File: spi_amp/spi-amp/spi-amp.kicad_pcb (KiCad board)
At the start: 4 copper layers, 22.3 x 32.8 mm, 5 parts, among them J1 IN+, J2 IN-, J3 OUT+, J4 OUT-, U1 LMH6401

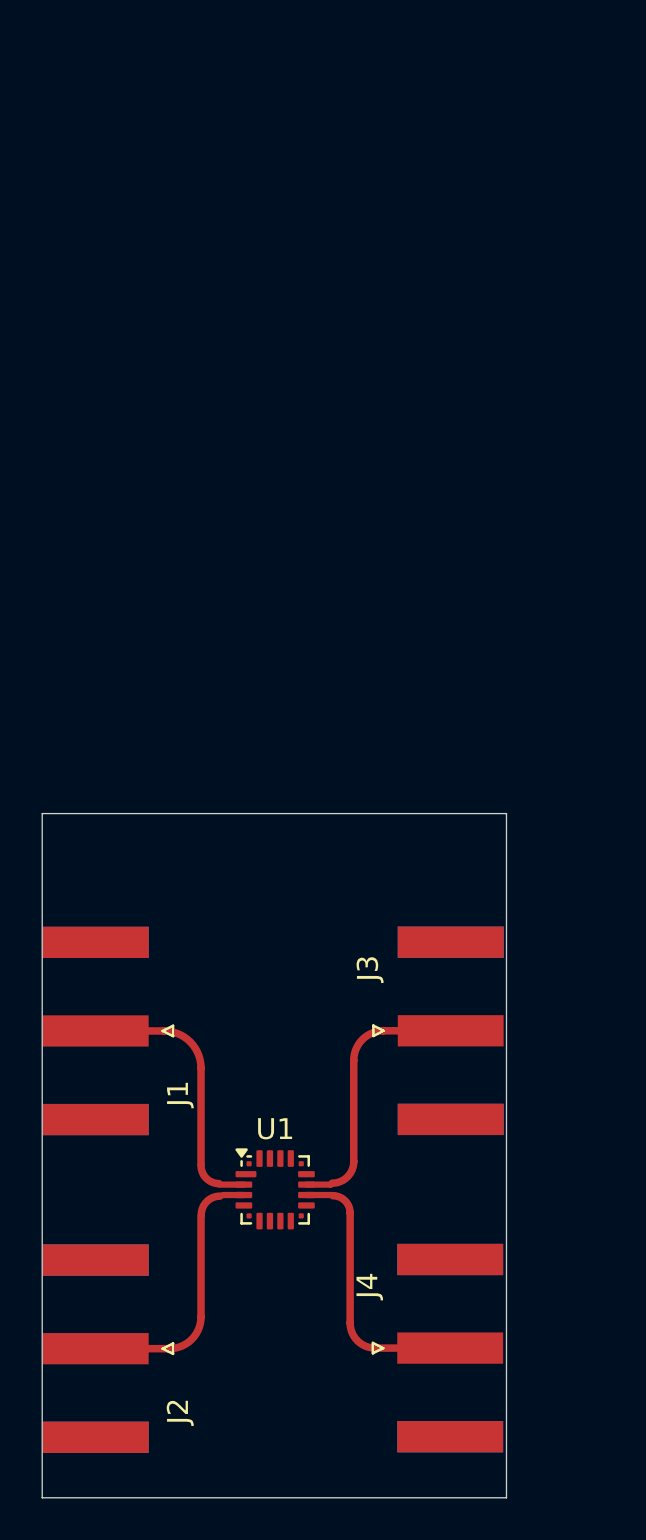
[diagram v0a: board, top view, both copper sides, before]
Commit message: Fixed layout for SPI RF PCB.
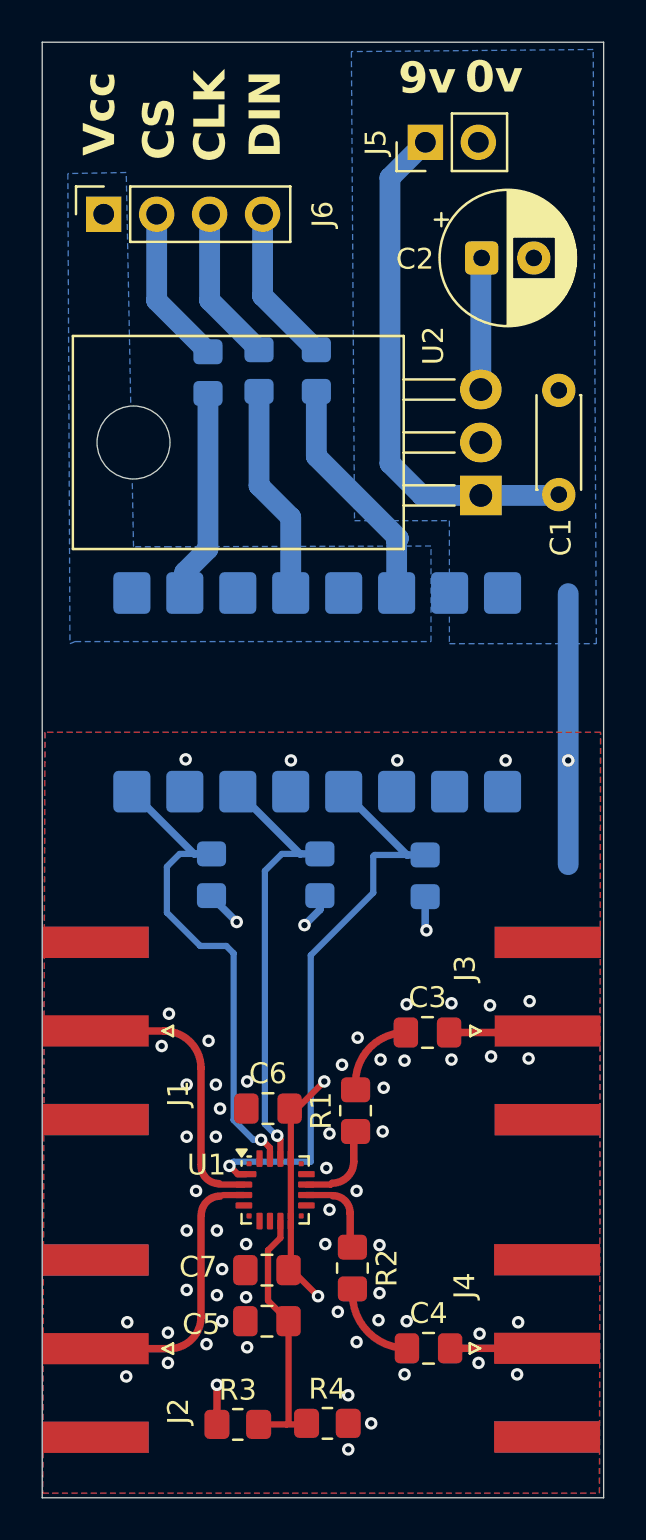
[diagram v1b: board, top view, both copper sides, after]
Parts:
- added C1: 47n, Capacitor_THT:C_Disc_D4.3mm_W1.9mm_P5.00mm, F.Cu at (130.7, 58.6)
- added C2: 22uF, Capacitor_THT:CP_Radial_D6.3mm_P2.50mm, F.Cu at (127.0, 47.2)
- added C3: 100n, Capacitor_SMD:C_0805_2012Metric_Pad1.18x1.45mm_HandSolder, F.Cu at (124.4, 84.4)
- added C4: 100n, Capacitor_SMD:C_0805_2012Metric_Pad1.18x1.45mm_HandSolder, F.Cu at (124.5, 99.5)
- added C5: 100n, Capacitor_SMD:C_0805_2012Metric_Pad1.18x1.45mm_HandSolder, F.Cu at (116.7, 98.2)
- added C6: 100n, Capacitor_SMD:C_0805_2012Metric_Pad1.18x1.45mm_HandSolder, F.Cu at (116.8, 88.0)
- added C7: 100n, Capacitor_SMD:C_0805_2012Metric_Pad1.18x1.45mm_HandSolder, F.Cu at (116.7, 95.8)
- added J5: Conn_01x02, Connector_PinHeader_2.54mm:PinHeader_1x02_P2.54mm_Vertical, F.Cu at (124.3, 41.7)
- added J6: Conn_01x04, Connector_PinSocket_2.54mm:PinSocket_1x04_P2.54mm_Vertical, F.Cu at (108.9, 45.1)
- added R1: 40, Resistor_SMD:R_0805_2012Metric_Pad1.20x1.40mm_HandSolder, F.Cu at (121.0, 88.2)
- added R10: 1.5k, Resistor_SMD:R_0805_2012Metric_Pad1.20x1.40mm_HandSolder, B.Cu at (124.3, 76.9)
- added R2: 40, Resistor_SMD:R_0805_2012Metric_Pad1.20x1.40mm_HandSolder, F.Cu at (120.8, 95.7)
- added R3: 1k, Resistor_SMD:R_0805_2012Metric_Pad1.20x1.40mm_HandSolder, F.Cu at (115.3, 103.2)
- added R4: 1k, Resistor_SMD:R_0805_2012Metric_Pad1.20x1.40mm_HandSolder, F.Cu at (119.6, 103.2)
- added R5: 1k, Resistor_SMD:R_0805_2012Metric_Pad1.20x1.40mm_HandSolder, B.Cu at (113.9, 52.8)
- added R6: 1k, Resistor_SMD:R_0805_2012Metric_Pad1.20x1.40mm_HandSolder, B.Cu at (116.3, 52.6)
- added R7: 1k, Resistor_SMD:R_0805_2012Metric_Pad1.20x1.40mm_HandSolder, B.Cu at (119.1, 52.6)
- added R8: 1.5k, Resistor_SMD:R_0805_2012Metric_Pad1.20x1.40mm_HandSolder, B.Cu at (114.0, 76.8)
- added R9: 1.5k, Resistor_SMD:R_0805_2012Metric_Pad1.20x1.40mm_HandSolder, B.Cu at (119.2, 76.8)
- added U2: LM78M05_TO220, Package_TO_SOT_THT:TO-220-3_Horizontal_TabDown, F.Cu at (127.0, 58.6)
- added U3: LTV-847S, Package_DIP:SMDIP-16_W9.53mm, B.Cu at (119.1, 68.1)
- moved J3 4.65 mm to (130.2, 84.3)
- moved J4 4.65 mm to (130.1, 99.5)
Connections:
- net Net-(U1-V+-Pad13) renamed VCC
- J1 pad 2: Net-(J1-Ext) -> DIG_GND
- J2 pad 2: Net-(J1-Ext) -> DIG_GND
- J3 pad 2: Net-(J1-Ext) -> DIG_GND
- J4 pad 2: Net-(J1-Ext) -> DIG_GND
- U1 pad 1: unconnected-(U1-SDI-Pad1) -> Net-(U1-SDI)
- U1 pad 10: Net-(J4-In) -> Net-(R2-Pad1)
- U1 pad 11: Net-(J3-In) -> Net-(R1-Pad1)
- U1 pad 12: Net-(J1-Ext) -> DIG_GND
- U1 pad 14: unconnected-(U1-CLK-Pad14) -> Net-(U1-CLK)
- U1 pad 15: unconnected-(U1-CS-Pad15) -> Net-(U1-CS)
- U1 pad 16: Net-(U1-V--Pad16) -> DIG_GND
- U1 pad 17: Net-(J1-Ext) -> DIG_GND
- U1 pad 5: Net-(U1-V--Pad16) -> DIG_GND
- U1 pad 6: unconnected-(U1-PD-Pad6) -> DIG_GND
- U1 pad 7: unconnected-(U1-NC-Pad7) -> Net-(U1-Vocm)
- U1 pad 9: Net-(J1-Ext) -> DIG_GND
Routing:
- net Net-(U1-SDI): track 0.00 -> 28.5 mm, vias 0 -> 1
- net VCC: track 0.00 -> 25.2 mm, vias 0 -> 6
- net Net-(J5-Pin_1): track 0.00 -> 24.9 mm
- net Net-(U1-CS): track 0.00 -> 24.5 mm, vias 0 -> 1
- net Net-(U1-CLK): track 0.00 -> 22.3 mm, vias 0 -> 1
- net DIG_GND: track 0.00 -> 13.1 mm, vias 0 -> 61
- net Net-(U1-Vocm): track 0.00 -> 12.8 mm
- net Net-(R7-Pad1): track 0.00 -> 11.3 mm
- net Net-(R6-Pad1): track 0.00 -> 10.3 mm
- net Net-(R5-Pad1): track 0.00 -> 10.0 mm
- net Net-(J4-In): track 13.3 -> 4.65 mm
- net Net-(J3-In): track 13.1 -> 4.75 mm
- net Net-(J6-Pin_2): track 0.00 -> 7.62 mm
- net Net-(J6-Pin_4): track 0.00 -> 7.57 mm
- net Net-(J6-Pin_3): track 0.00 -> 7.48 mm
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- added copper zone on B.Cu, net DIG_GND
- added copper zone on F.Cu, net DIG_GND
- added copper zone on In1.Cu, net DIG_GND
- added copper zone on B.Cu, net LED_VCC
- added copper zone on In2.Cu, net VCC
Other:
- board size 22.3 x 32.8 mm -> 26.9 x 69.8 mm
- board text added: "0v"
- board text added: "9v"
- board text added: "CLK"
- board text added: "CS"
- board text added: "DIN"
- board text added: "Vcc"
